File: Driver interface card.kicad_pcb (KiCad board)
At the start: 2 copper layers, 128.8 x 78 mm, 68 parts, among them J1 Motor 1, J2 V IN, J3 V OUT, J6 Motor 2, J7 395026004, J8 395021010, J9 395021010, Q1 2N7002H, Q2 2N7002H, Q3 2N7002H, Q4 2N7002H, Q5 2N7002H, Q6 2N7002H, Q7 2N7002H, Q8 2N7002H, SW1 SW_DPST_x2, SW2 SW_DPST_x2, U1 XL1509-5.0

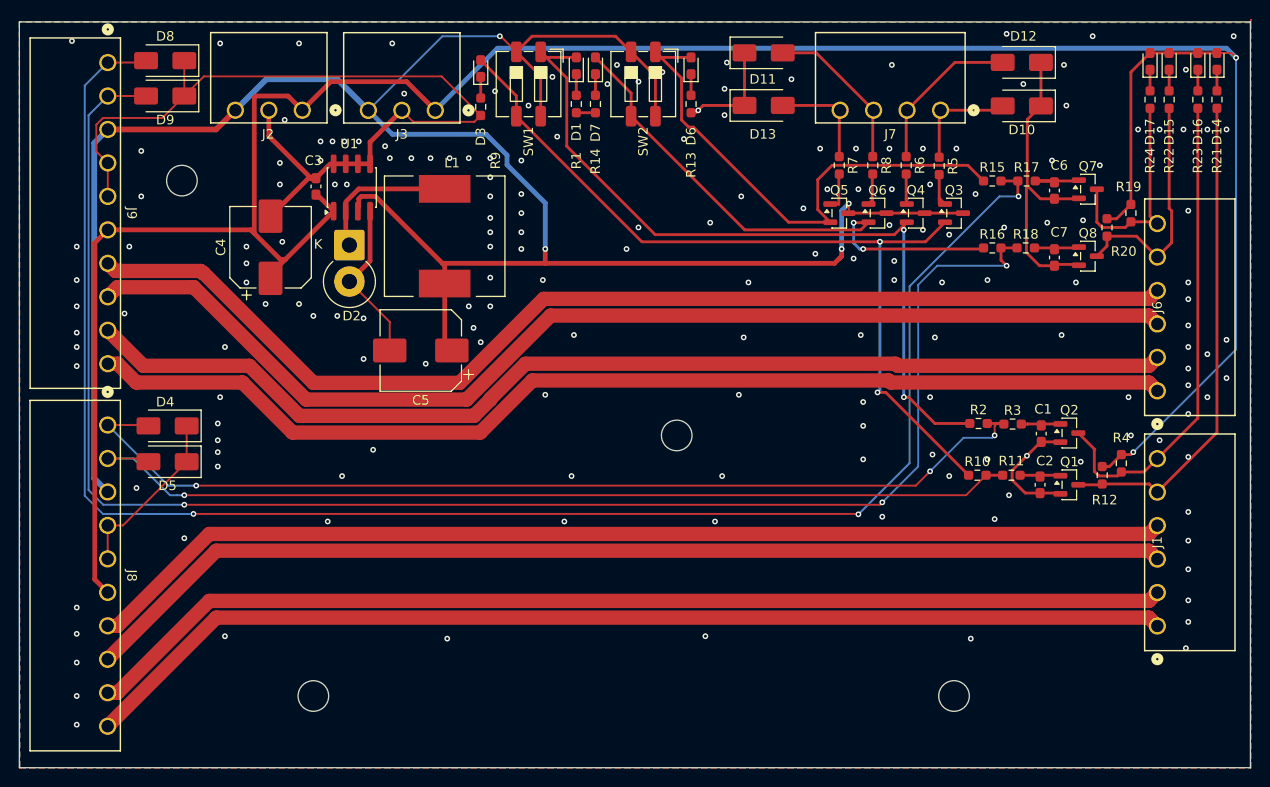
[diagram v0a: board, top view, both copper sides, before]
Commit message: rev2
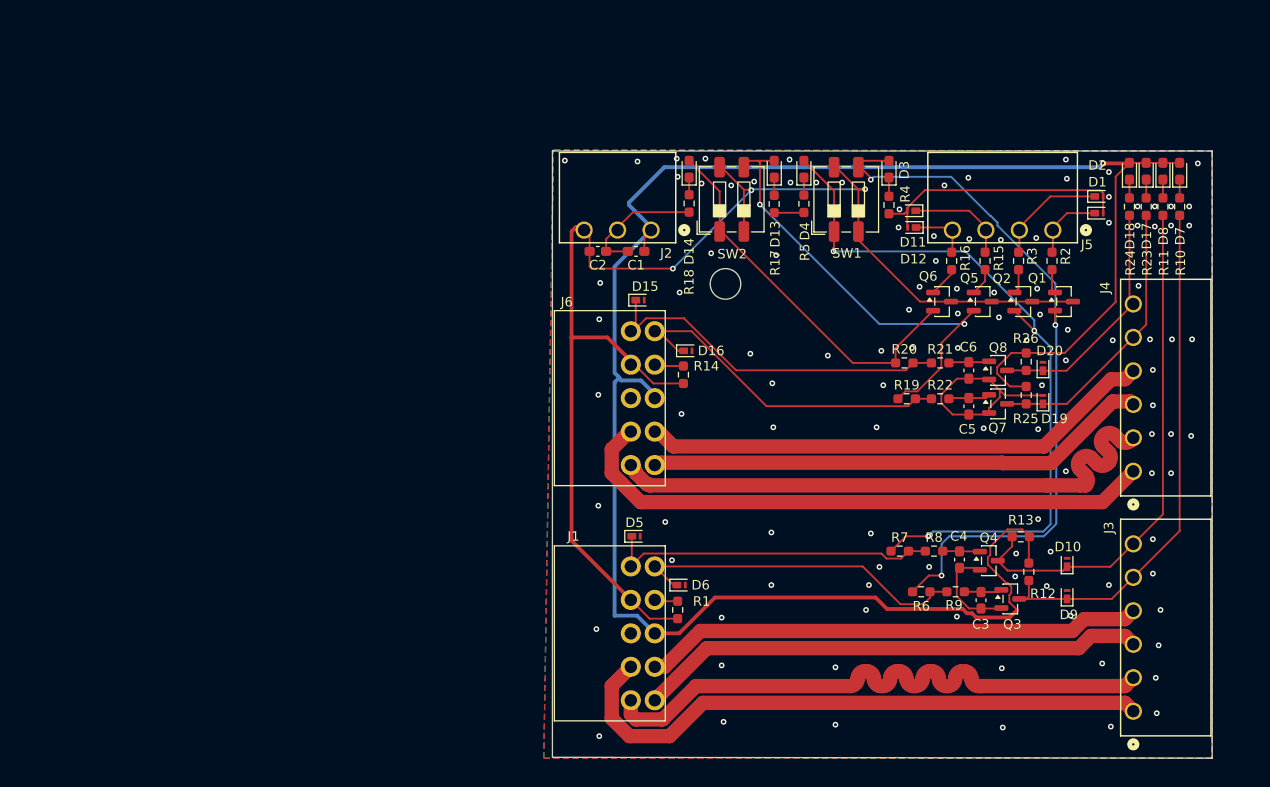
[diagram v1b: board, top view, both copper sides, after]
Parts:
- removed ?: LOGO, footprints:eli logo 1 cm
- removed C7: 0u1, Capacitor_SMD:C_0603_1608Metric_Pad1.08x0.95mm_HandSolder
- removed J7: 395026004, MOLEX:CONN_SD-39502-001_04P_MOL
- removed J8, J9: 395021010, MOLEX:CONN_SD-39502-001_10P_MOL
- removed L1: 68uH/2A, Inductor_SMD:L_12x12mm_H6mm
- removed U1: XL1509-5.0, Package_SO:SOIC-8_3.9x4.9mm_P1.27mm
- added D18: LED, LED_SMD:LED_0603_1608Metric_Pad1.05x0.95mm_HandSolder, F.Cu at (205.8, 57.1)
- added D19: PTVS26VZ1USK, Diode_SMD:Nexperia_DSN1608-2_1.6x0.8mm, F.Cu at (196.8, 81.2)
- added D20: PTVS26VZ1USK, Diode_SMD:Nexperia_DSN1608-2_1.6x0.8mm, F.Cu at (196.8, 77.7)
- added G***: LOGO, footprints:eli logo 1 cm, B.Cu at (185.3, 92.8)
- added J4: Motor 2, MOLEX:CONN_SD-39502-001_06P_MOL, F.Cu at (206.2, 88.5)
- added J5: 395026004, MOLEX:CONN_SD-39502-001_04P_MOL, F.Cu at (197.8, 63.3)
- added R25: 8k2, Resistor_SMD:R_0603_1608Metric_Pad0.98x0.95mm_HandSolder, F.Cu at (195.1, 80.5)
- added R26: 8k2, Resistor_SMD:R_0603_1608Metric_Pad0.98x0.95mm_HandSolder, F.Cu at (195.1, 77.0)
- C1, C2: value 0u1 -> 1u
- C3: value 1u -> 0u1
- C4: value 470u -> 0u1; footprint Capacitor_SMD:CP_Elec_8x10 -> Capacitor_SMD:C_0603_1608Metric_Pad1.08x0.95mm_HandSolder
- C5: value 180u -> 0u1; footprint Capacitor_SMD:CP_Elec_8x10 -> Capacitor_SMD:C_0603_1608Metric_Pad1.08x0.95mm_HandSolder
- D1, D15, D16, D6: value LED -> PTVS26VZ1USK; footprint LED_SMD:LED_0603_1608Metric_Pad1.05x0.95mm_HandSolder -> Diode_SMD:Nexperia_DSN1608-2_1.6x0.8mm
- D10, D11, D12, D5, D9: value SMAJ26CA -> PTVS26VZ1USK; footprint Diode_SMD:D_SMA -> Diode_SMD:Nexperia_DSN1608-2_1.6x0.8mm
- D13, D4, D8: value SMAJ26CA -> LED; footprint Diode_SMD:D_SMA -> LED_SMD:LED_0603_1608Metric_Pad1.05x0.95mm_HandSolder
- D2: value SS34 -> PTVS26VZ1USK; footprint Diode_THT:D_DO-201AD_P3.81mm_Vertical_KathodeUp -> Diode_SMD:Nexperia_DSN1608-2_1.6x0.8mm
- J1: value Motor 1 -> Conn_02x05_Counter_Clockwise; footprint MOLEX:CONN_SD-39502-001_06P_MOL -> footprints:DMC 1,5 5-G1-3,5 P20THR
- J3: value V OUT -> Motor 1; footprint MOLEX:CONN_SD-39502-001_03P_MOL -> MOLEX:CONN_SD-39502-001_06P_MOL
- J6: value Motor 2 -> Conn_02x05_Counter_Clockwise; footprint MOLEX:CONN_SD-39502-001_06P_MOL -> footprints:DMC 1,5 5-G1-3,5 P20THR
- R1, R14: value 1k5 -> 10k
- R10: value 10k -> 4k3
- R11: value 1k -> 4k3
- R13: value 1k5 -> 8k2
- R17, R18: value 1k -> 1k5
- R19, R20: value 8k2 -> 10k
- R21, R22: value 2k5 -> 1k
- R23, R24: value 2k5 -> 4k3
- R3: value 1k -> 10k
- R4: value 8k2 -> 1k5
- R5: value 10k -> 1k5
- R8: value 10k -> 1k
- R9: value 1k5 -> 1k
- moved D9 107.9 mm to (199.3, 101.6), turned to 90 degrees
- moved D8 105.0 mm to (209.3, 57.1), turned to 90 degrees
- moved J3 96.3 mm to (206.2, 113.6), turned to 90 degrees
- moved C3 81.9 mm to (190.3, 102.0), turned to -90 degrees
- moved C4 79.1 mm to (188.1, 97.7), turned to -90 degrees
- moved D2 78.4 mm to (202.5, 59.8), turned to 0 degrees
- moved D4 71.8 mm to (171.8, 56.9), turned to 90 degrees
- moved R9 71.0 mm to (187.7, 101.1), turned to 0 degrees
- moved D7 62.1 mm to (211.1, 57.1)
- moved D16 61.5 mm to (159.5, 75.9), turned to 0 degrees
- moved D15 60.9 mm to (154.5, 70.6), turned to 0 degrees
- moved C5 57.6 mm to (189.1, 81.7), turned to -90 degrees
- moved J1 57.4 mm to (151.4, 105.3), turned to 180 degrees
- moved J6 57.4 mm to (151.4, 80.7), turned to 180 degrees
- moved R13 56.9 mm to (194.5, 95.3), turned to 180 degrees
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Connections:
- C1 pad 1: Net-(Q2-G) -> VCC
- C2 pad 1: Net-(Q1-G) -> GND
- C2 pad 2: GND -> 5V
- C3 pad 1: VCC -> Net-(Q3-G)
- C4 pad 1: VCC -> Net-(Q4-G)
- C5 pad 1: 5V -> Net-(Q7-G)
- C6 pad 1: Net-(Q7-G) -> Net-(Q8-G)
- D1 pad 1: Net-(D1-K) -> /Driver connector/Home1Pullup
- D1 pad 2: Net-(D1-A) -> GND
- D10 pad 1: GND -> /Driver connector/LimitOUT1.End
- D10 pad 2: /Driver connector/Home1Pullup -> GND
- D11 pad 1: GND -> /Driver connector/Home2Pullup
- D11 pad 2: /Driver connector/Home2Pullup -> GND
- D12 pad 1: GND -> /Driver connector/End2Pullup
- D12 pad 2: /Driver connector/End1Pullup -> GND
- D13 pad 1: GND -> Net-(D13-K)
- D13 pad 2: /Driver connector/End2Pullup -> Net-(D13-A)
- D14 pad 2: VCC -> Net-(D14-A)
- D15 pad 1: Net-(D15-K) -> /Logic converter1/LimitIN.End
- D15 pad 2: VCC -> GND
- D16 pad 1: Net-(D16-K) -> /Logic converter1/LimitIN.Home
- D16 pad 2: VCC -> GND
- D2 pad 1: Net-(D2-K) -> /Driver connector/End1Pullup
- D4 pad 1: GND -> Net-(D4-K)
- D4 pad 2: /Logic converter/LimitIN.End -> Net-(D4-A)
- D5 pad 1: GND -> /Logic converter/LimitIN.End
- D5 pad 2: /Logic converter/LimitIN.Home -> GND
- D6 pad 1: Net-(D6-K) -> /Logic converter/LimitIN.Home
- D6 pad 2: Net-(D6-A) -> GND
- D7 pad 2: Net-(D7-A) -> VCC
- D8 pad 1: GND -> Net-(D8-K)
- D8 pad 2: /Logic converter1/LimitIN.End -> VCC
- D9 pad 1: GND -> /Driver connector/LimitOUT1.Home
- D9 pad 2: /Logic converter1/LimitIN.Home -> GND
- J1 pad 1: /Driver connector/Phase1.A+ -> /Logic converter/LimitIN.Home
- J1 pad 2: /Driver connector/Phase1.A- -> Net-(J1-Pin_2)
- J1 pad 3: /Driver connector/Phase1.B+ -> VCC
- J1 pad 5: /Driver connector/LimitOUT1.Home -> /Driver connector/Phase1.B+
- J1 pad 6: /Driver connector/LimitOUT1.End -> /Driver connector/Phase1.A-
- J3 pad 1: VCC -> /Driver connector/Phase1.A+
- J3 pad 2: GND -> /Driver connector/Phase1.A-
- J3 pad 3: 5V -> /Driver connector/Phase1.B+
- J6 pad 1: /Driver connector/Phase2.A+ -> /Logic converter1/LimitIN.Home
- J6 pad 2: /Driver connector/Phase2.A- -> Net-(J6-Pin_2)
- J6 pad 3: /Driver connector/Phase2.B+ -> VCC
- J6 pad 5: /Driver connector/LimitOUT2.Home -> /Driver connector/Phase2.B+
- J6 pad 6: /Driver connector/LimitOUT2.End -> /Driver connector/Phase2.A-
- Q1 pad 2: GND -> Net-(D3-A)
- Q1 pad 3: /Driver connector/LimitOUT1.Home -> 5V
- Q2 pad 2: GND -> Net-(D4-A)
- Q2 pad 3: /Driver connector/LimitOUT1.End -> 5V
- Q3 pad 2: Net-(D3-A) -> GND
- Q3 pad 3: 5V -> /Driver connector/LimitOUT1.Home
- Q4 pad 2: Net-(D1-A) -> GND
- Q4 pad 3: 5V -> /Driver connector/LimitOUT1.End
- Q5 pad 2: Net-(D6-A) -> Net-(D13-A)
- Q6 pad 2: Net-(D7-A) -> Net-(D14-A)
- Q7 pad 3: /Driver connector/LimitOUT2.End -> /Driver connector/LimitOUT2.Home
- Q8 pad 3: /Driver connector/LimitOUT2.Home -> /Driver connector/LimitOUT2.End
- R1 pad 1: Net-(D1-K) -> 5V
- R1 pad 2: GND -> Net-(J1-Pin_2)
- R10 pad 1: Net-(D3-A) -> Net-(D7-K)
- R10 pad 2: /Logic converter/LimitIN.Home -> /Driver connector/LimitOUT1.Home
- R11 pad 1: /Logic converter/LimitIN.Home -> Net-(D8-K)
- R11 pad 2: Net-(Q1-G) -> /Driver connector/LimitOUT1.End
- R13 pad 1: Net-(D6-K) -> VCC
- R13 pad 2: GND -> /Driver connector/LimitOUT1.End
- R14 pad 1: Net-(D7-K) -> 5V
- R14 pad 2: GND -> Net-(J6-Pin_2)
- R15 pad 1: Net-(D6-A) -> /Driver connector/Home2Pullup
- R15 pad 2: /Logic converter1/LimitIN.End -> Net-(Q5-G)
- R16 pad 1: Net-(D7-A) -> /Driver connector/End2Pullup
- R16 pad 2: /Logic converter1/LimitIN.Home -> Net-(Q6-G)
- R17 pad 1: /Logic converter1/LimitIN.End -> Net-(D13-K)
- R17 pad 2: Net-(Q7-G) -> GND
- R18 pad 1: /Logic converter1/LimitIN.Home -> Net-(D14-K)
- R18 pad 2: Net-(Q8-G) -> GND
- R19 pad 1: VCC -> Net-(D13-A)
- R19 pad 2: /Driver connector/LimitOUT2.End -> /Logic converter1/LimitIN.Home
- R2 pad 1: Net-(D1-A) -> /Driver connector/Home1Pullup
- R2 pad 2: /Logic converter/LimitIN.End -> Net-(Q1-G)
- R20 pad 1: VCC -> Net-(D14-A)
- R20 pad 2: /Driver connector/LimitOUT2.Home -> /Logic converter1/LimitIN.End
- R21 pad 1: Net-(D14-K) -> /Logic converter1/LimitIN.End
- R21 pad 2: /Driver connector/LimitOUT1.Home -> Net-(Q8-G)
- R22 pad 1: Net-(D15-K) -> /Logic converter1/LimitIN.Home
- R22 pad 2: /Driver connector/LimitOUT2.Home -> Net-(Q7-G)
- R23 pad 1: Net-(D16-K) -> Net-(D17-K)
- R23 pad 2: /Driver connector/LimitOUT1.End -> /Driver connector/LimitOUT2.Home
- R24 pad 1: Net-(D17-K) -> Net-(D18-K)
- R3 pad 1: /Logic converter/LimitIN.End -> /Driver connector/End1Pullup
- R4 pad 1: VCC -> Net-(D3-K)
- R4 pad 2: /Driver connector/LimitOUT1.End -> GND
- R5 pad 1: /Driver connector/Home1Pullup -> Net-(D4-K)
- R5 pad 2: Net-(Q3-G) -> GND
- R6 pad 1: /Driver connector/End1Pullup -> Net-(D3-A)
- R6 pad 2: Net-(Q4-G) -> /Logic converter/LimitIN.Home
- R7 pad 1: /Driver connector/End2Pullup -> Net-(D4-A)
- R7 pad 2: Net-(Q5-G) -> /Logic converter/LimitIN.End
- R8 pad 1: /Driver connector/Home2Pullup -> /Logic converter/LimitIN.End
- R8 pad 2: Net-(Q6-G) -> Net-(Q4-G)
- R9 pad 1: Net-(D3-K) -> /Logic converter/LimitIN.Home
- R9 pad 2: GND -> Net-(Q3-G)
- SW1 pad 1: Net-(D1-A) -> Net-(D4-A)
- SW2 pad 1: Net-(D6-A) -> Net-(D14-A)
- SW2 pad 3: Net-(D7-A) -> Net-(D13-A)
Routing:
- net /Logic converter1/LimitIN.End: track 176.9 -> 37.2 mm, vias 3 -> 0
- net /Logic converter1/LimitIN.Home: track 168.0 -> 35.6 mm, vias 3 -> 0
- net GND: track 187.7 -> 76.2 mm, vias 182 -> 113
- net 5V: track 231.0 -> 142.1 mm, vias 4 -> 3
- net Net-(D1-A): track 80.9 -> 0.00 mm, vias 2 -> 0
- net Net-(D4-A): track 0.00 -> 77.6 mm, vias 0 -> 3
- net /Logic converter/LimitIN.End: track 105.0 -> 35.1 mm, vias 3 -> 0
- net /Driver connector/Phase2.B+: track 119.0 -> 53.0 mm
- net /Driver connector/Phase2.B-: track 118.9 -> 54.0 mm
- net /Logic converter/LimitIN.Home: track 100.5 -> 36.2 mm, vias 1 -> 0
- net VCC: track 272.9 -> 209.5 mm, vias 2 -> 1
- net /Driver connector/Phase1.B-: track 114.1 -> 52.5 mm
- net /Driver connector/Phase1.B+: track 114.8 -> 53.2 mm
- net Net-(D6-A): track 55.8 -> 0.00 mm
- net Net-(D7-A): track 55.4 -> 0.00 mm, vias 2 -> 0
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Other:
- board size 128.8 x 78 mm -> 69 x 63.5 mm
- board text added: "5V"
- board text added: "5V* - 10k pullup to 5V"
- board text added: "A+ A- B+ B- HOME END"
- board text added: "GND"
- board text added: "HOME END HOME END"
- board text added: "HOME Motor 1 END HOME Motor 2 END"
- board text added: "M1 M2"
- board text added: "MOTOR 1 IN"
- board text added: "MOTOR 2 IN"
- board text added: "MTR 1 OUT"
- board text added: "MTR 2 OUT"
- board text added: "Manual pullup & status"
- board text added: "Motor interface board Rev 2"
- board text added: "Power IN"
- board text added: "Remote pullup"
- board text added: "VCC"
- board text removed: "L4b Driver interface board REV. 1"
